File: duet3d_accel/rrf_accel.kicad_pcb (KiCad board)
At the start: 2 copper layers, 118.7 x 50.3 mm, 13 parts, among them J1 Conn_02x05_Odd_Even, U1 LIS3DH

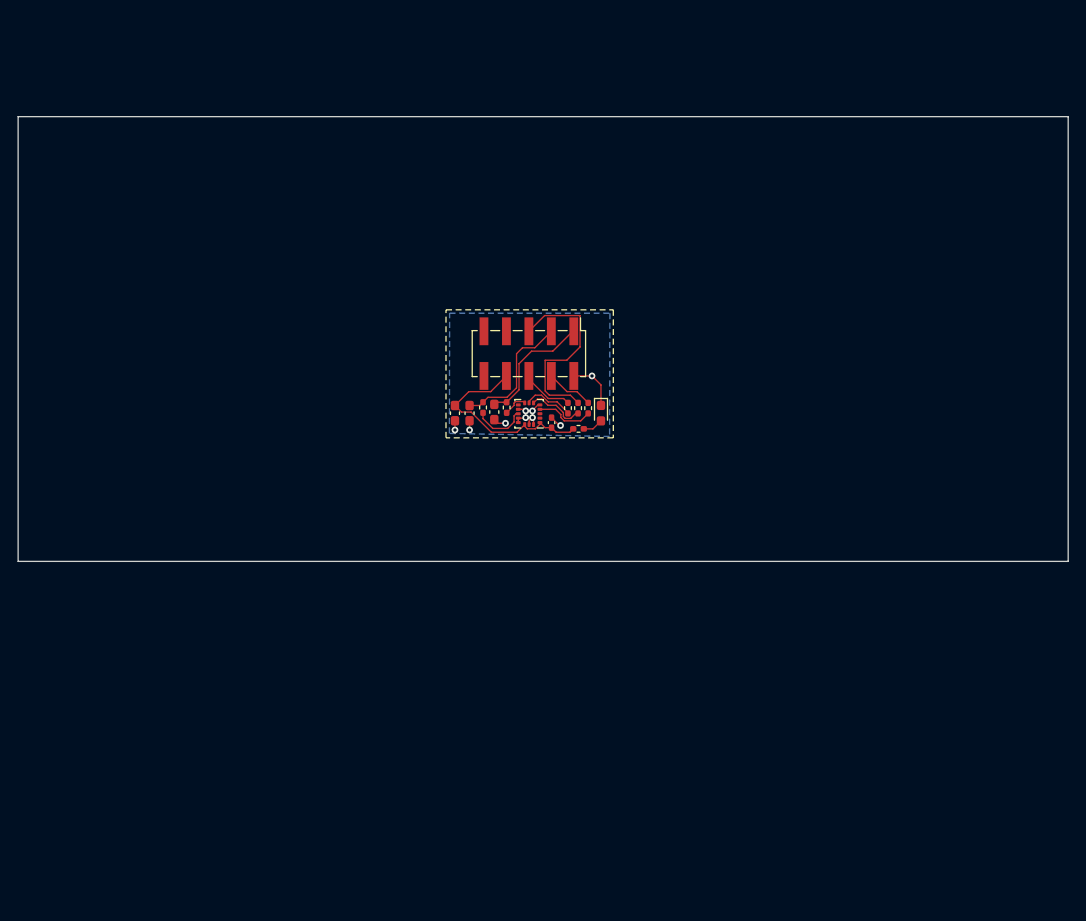
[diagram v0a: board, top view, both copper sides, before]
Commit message: Layout in progress.
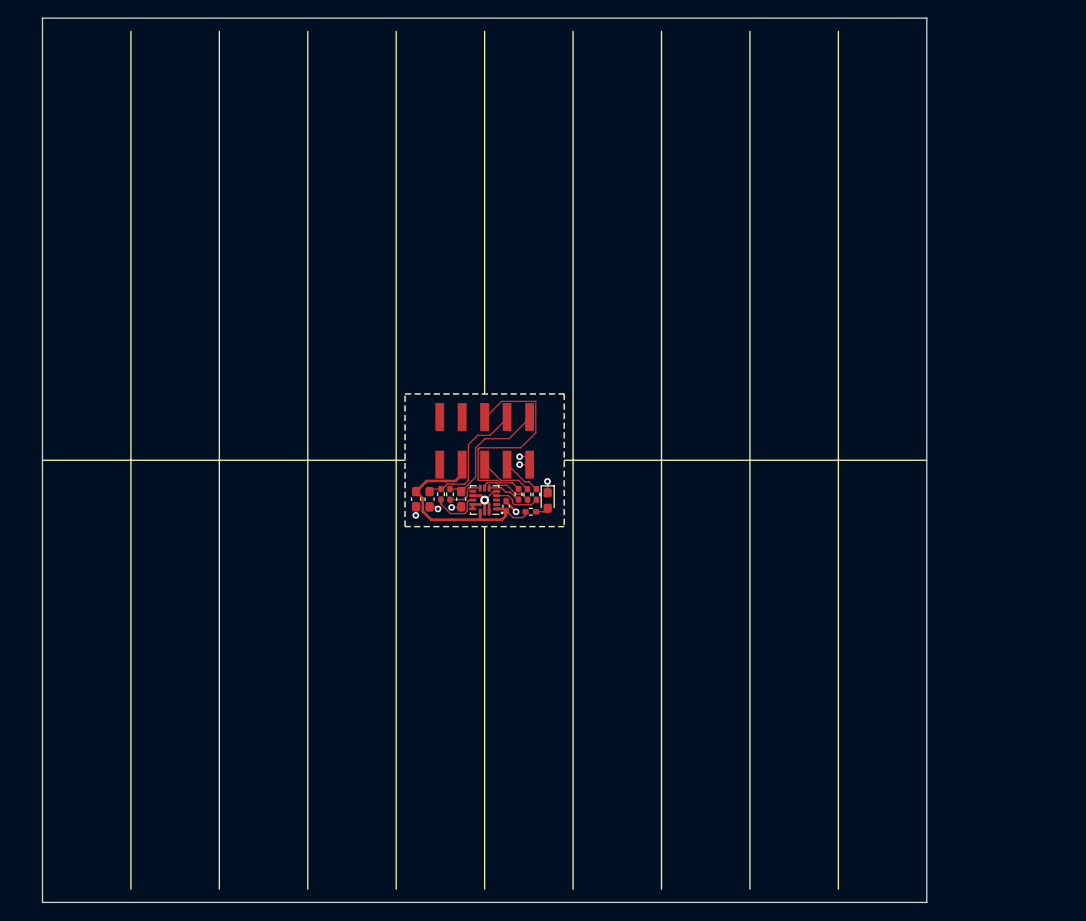
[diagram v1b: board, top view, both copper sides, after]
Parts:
- U1: footprint Package_LGA:LGA-16_3x3mm_P0.5mm_LayoutBorder3x5y -> duet3d_accel:LGA-16_3x3mm_P0.5mm_LayoutBorder3x5y
- moved R4 11.8 mm to (103.8, 99.3)
- moved R6 11.7 mm to (96.1, 99.4)
- moved D1 11.6 mm to (107.1, 100.1)
- moved R5 11.4 mm to (105.9, 99.4)
- moved J1 11.1 mm to (100.0, 93.3)
- moved U1 11.0 mm to (100.0, 100.0)
- moved R1 10.9 mm to (95.1, 99.3)
- moved R3 10.8 mm to (105.2, 101.3)
- moved R2 10.8 mm to (104.8, 99.4)
- moved C2 10.8 mm to (102.4, 100.7)
- moved C3 10.7 mm to (93.8, 99.9)
- moved C1 10.7 mm to (92.2, 99.9)
- moved C4 10.5 mm to (97.3, 99.9)
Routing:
- net /MOSI: track 22.4 -> 26.0 mm
- net Net-(U1-SDA/SDI/SDO): track 6.61 -> 3.88 mm
- net +3V3: track 23.5 -> 25.2 mm
- net Net-(U1-CS): track 2.79 -> 4.40 mm
- net Net-(U1-SCL/SPC): track 6.54 -> 5.48 mm
- net /SCK: track 5.43 -> 4.53 mm
- net Net-(D1-A): track 2.32 -> 1.47 mm
- net /CS: track 14.1 -> 14.8 mm
- net /INT: track 15.0 -> 14.5 mm
- net GNDD: track 16.6 -> 16.4 mm, vias 9 -> 8
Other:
- board size 118.7 x 50.3 mm -> 100 x 100 mm
